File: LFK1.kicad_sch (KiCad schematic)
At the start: 22 parts, among them J1 AVR-ISP-6, U1 ATmega32U4-A, U2 PRTR5V0U2X, Y1 Crystal_GND24_Small

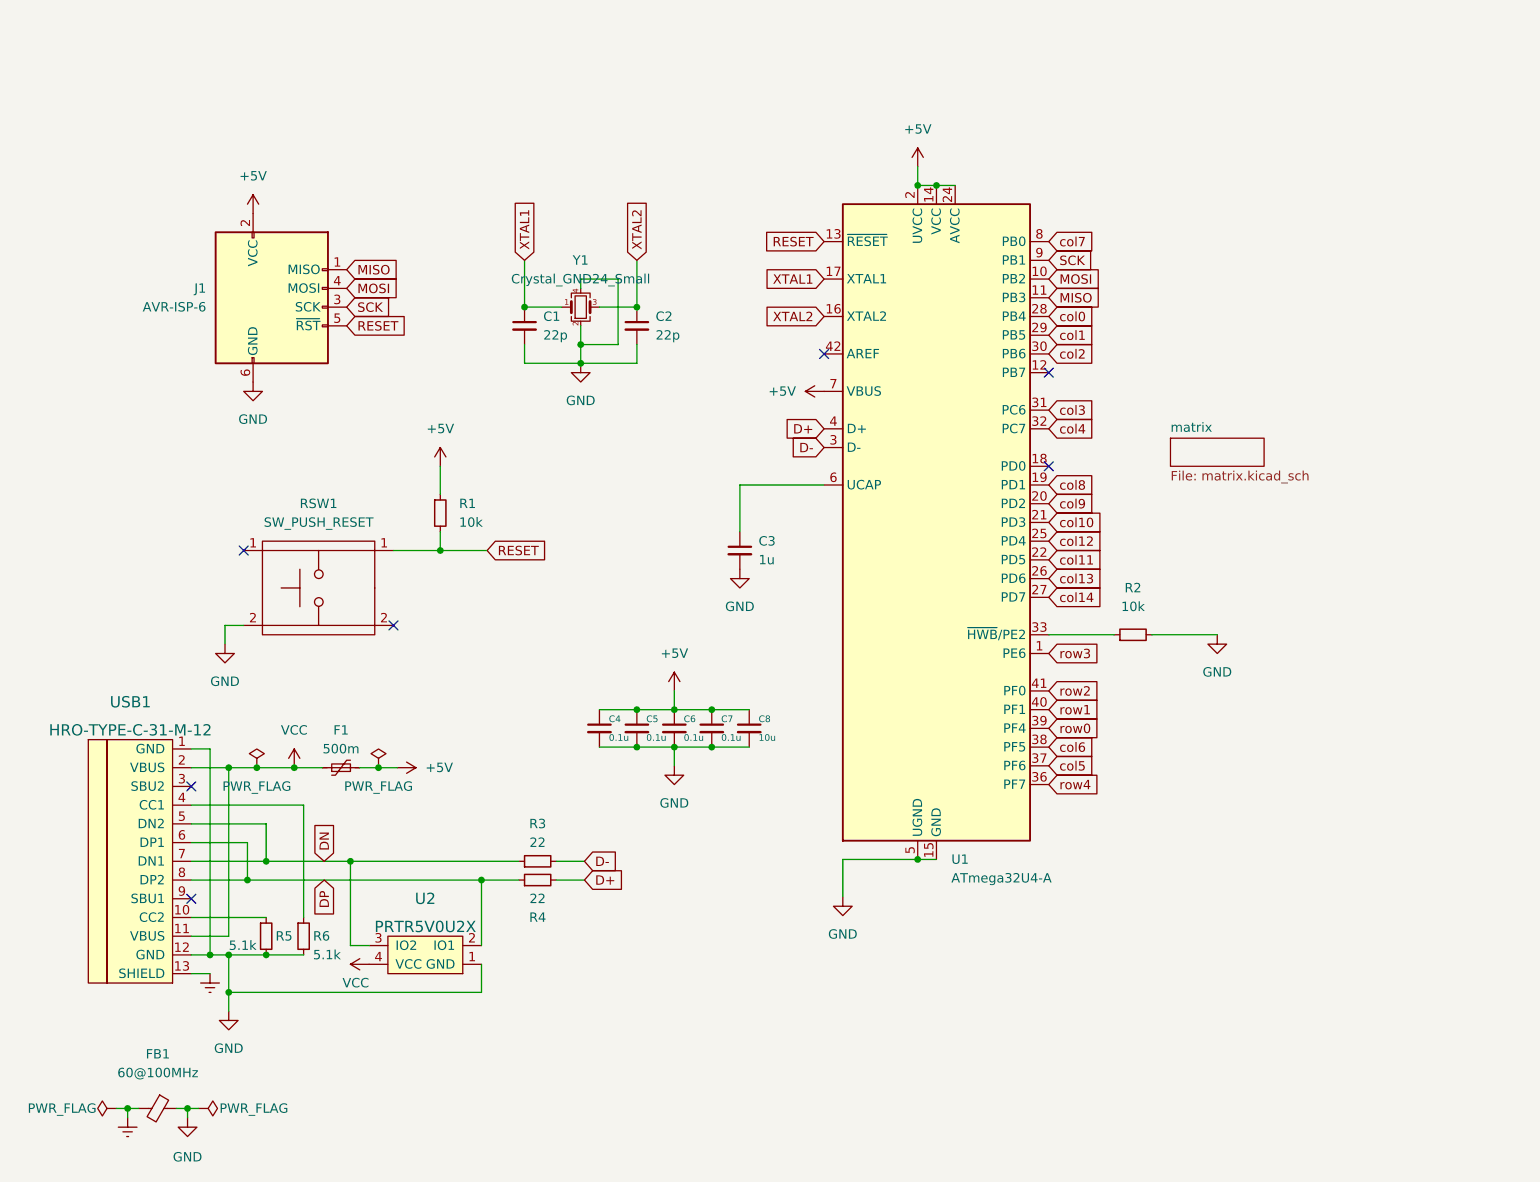
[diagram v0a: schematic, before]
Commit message: routing
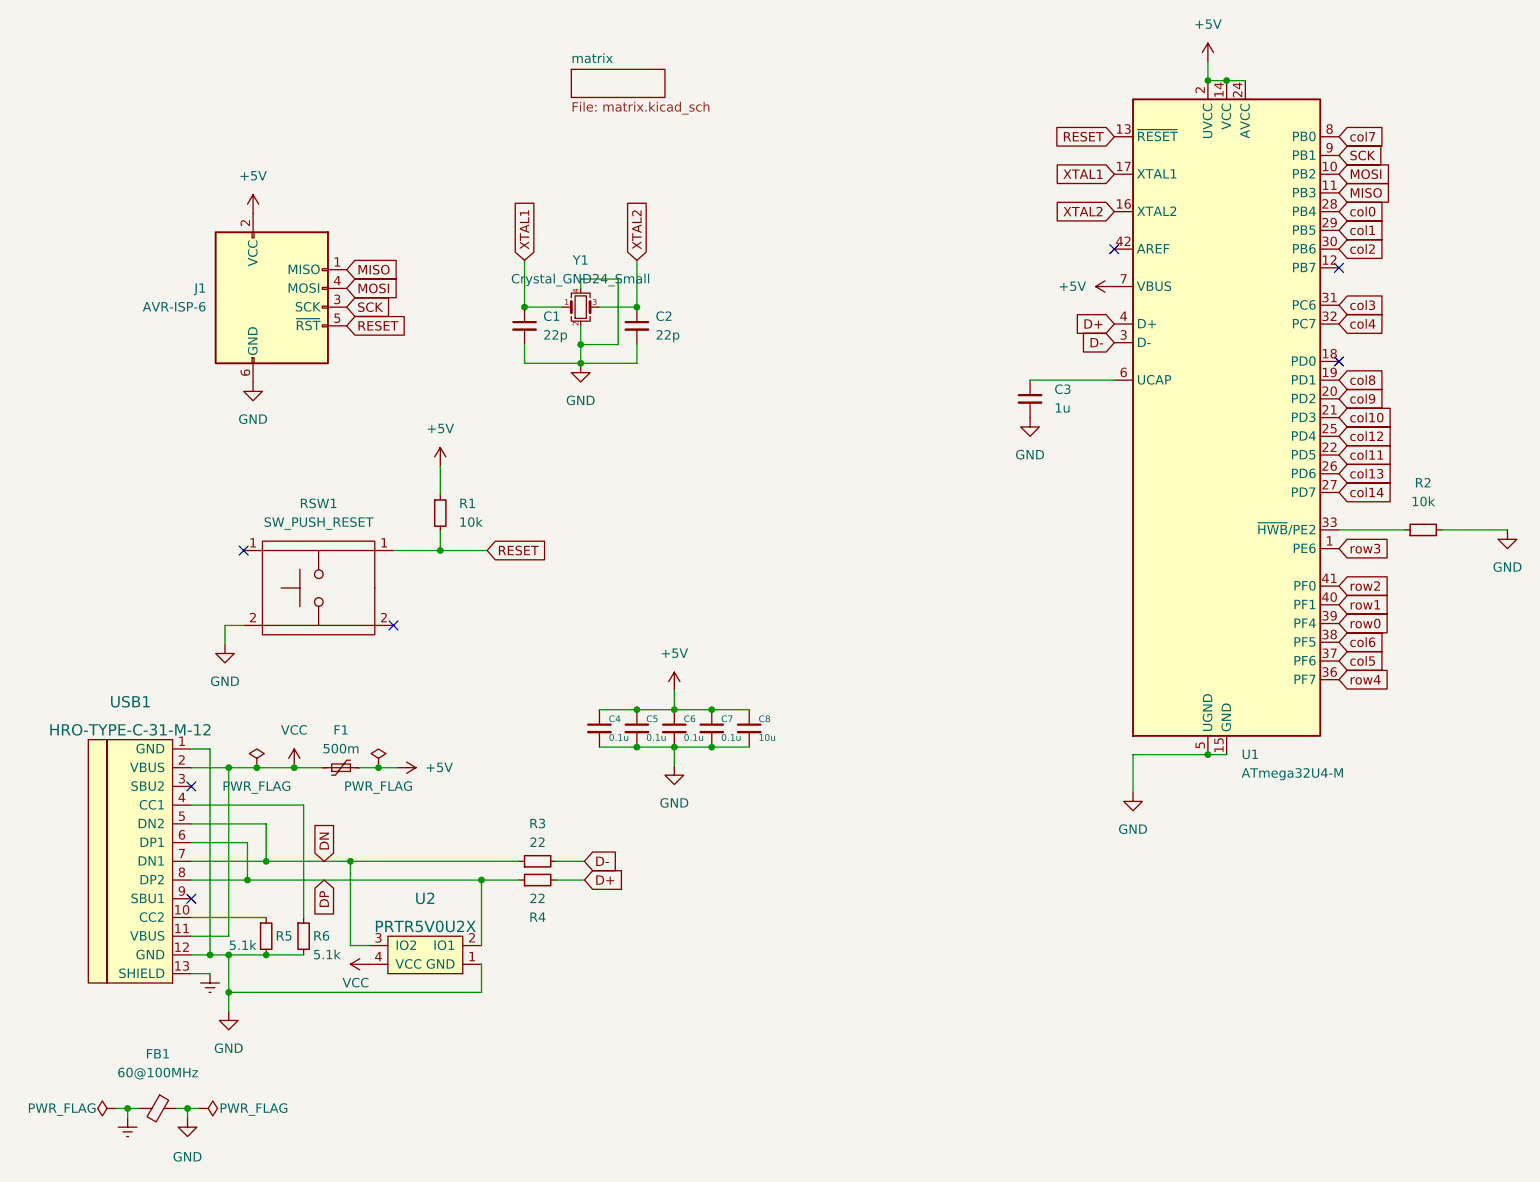
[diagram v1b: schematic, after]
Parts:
- removed U1: ATmega32U4-A, Package_QFP:TQFP-44_10x10mm_P0.8mm, symbol MCU_Microchip_ATmega:ATmega32U4-A
- added U1: ATmega32U4-M, Package_DFN_QFN:QFN-44-1EP_7x7mm_P0.5mm_EP5.2x5.2mm, symbol MCU_Microchip_ATmega:ATmega32U4-M
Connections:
- net +5V: now also U1.14 (VCC), U1.2 (UVCC), U1.24 (AVCC), U1.34 (VCC), U1.44 (AVCC), U1.7 (VBUS)
- net D+: now also U1.4 (D+)
- net D-: now also U1.3 (D-)
- net GND: now also U1.15 (GND), U1.23 (GND), U1.35 (GND), U1.43 (GND), U1.45 (GND), U1.5 (UGND)
- net MISO: now also U1.11 (PB3)
- net MOSI: now also U1.10 (PB2)
- net RESET: now also U1.13 (~{RESET})
- net SCK: now also U1.9 (PB1)
- net XTAL1: now also U1.17 (XTAL1)
- net XTAL2: now also U1.16 (XTAL2)
- net col0: now also U1.28 (PB4)
- net col1: now also U1.29 (PB5)
- net col10: now also U1.21 (PD3)
- net col11: now also U1.22 (PD5)
- net col12: now also U1.25 (PD4)
- net col13: now also U1.26 (PD6)
- net col14: now also U1.27 (PD7)
- net col2: now also U1.30 (PB6)
- net col3: now also U1.31 (PC6)
- net col4: now also U1.32 (PC7)
- net col5: now also U1.37 (PF6)
- net col6: now also U1.38 (PF5)
- net col7: now also U1.8 (PB0)
- net col8: now also U1.19 (PD1)
- net col9: now also U1.20 (PD2)
- net row0: now also U1.39 (PF4)
- net row1: now also U1.40 (PF1)
- net row2: now also U1.41 (PF0)
- net row3: now also U1.1 (PE6)
- net row4: now also U1.36 (PF7)
- net at R2.1: now also U1.33 (~{HWB}/PE2)
- net at C3.1: now also U1.6 (UCAP)
